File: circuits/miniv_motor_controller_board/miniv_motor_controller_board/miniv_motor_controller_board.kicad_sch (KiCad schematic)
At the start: 25 parts, among them J1 DC_in, J2 T200_ESC_power, J3 T200_ESC_signal, J4 Conn_EStop_Signal, Q1 2SC1815, Q2 2SC1815, U1 Teensy4.1, U2 TLP222A, U3 TLP222A

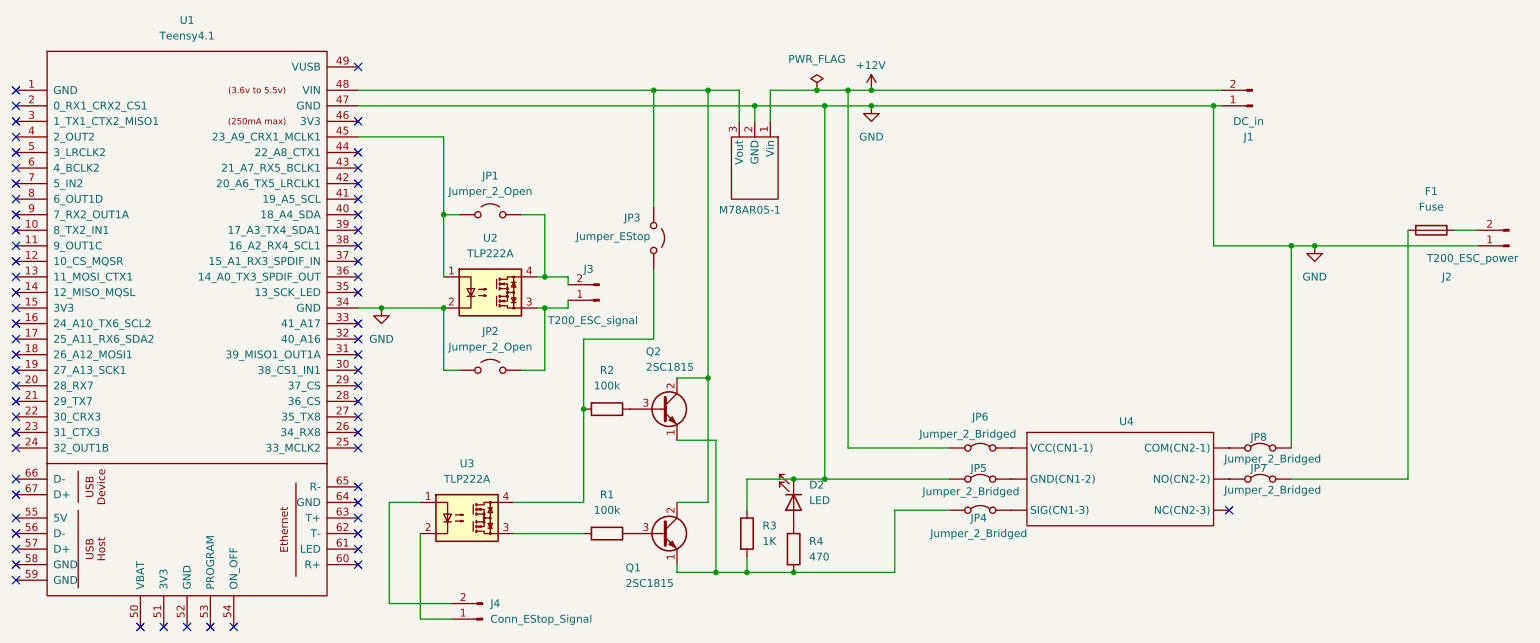
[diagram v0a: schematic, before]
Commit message: modify resister
Signed-off-by: Masaya Kataoka <ms.kataoka@gmail.com>
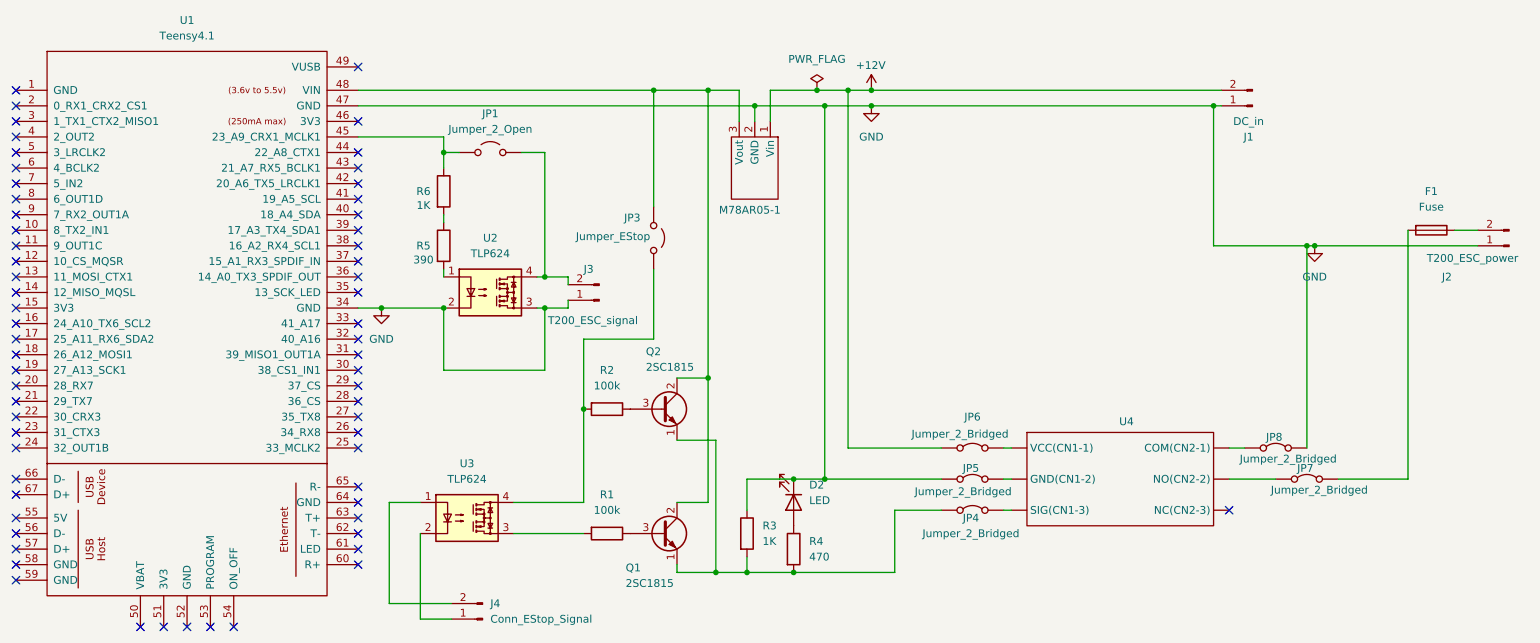
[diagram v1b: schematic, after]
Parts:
- removed JP2: Jumper_2_Open, Connector_PinHeader_2.54mm:PinHeader_1x02_P2.54mm_Vertical, symbol Jumper:Jumper_2_Open
- added R5: 390, Resistor_THT:R_Axial_DIN0207_L6.3mm_D2.5mm_P10.16mm_Horizontal, symbol Device:R
- added R6: 1K, Resistor_THT:R_Axial_DIN0207_L6.3mm_D2.5mm_P10.16mm_Horizontal, symbol Device:R
- J3: footprint (none) -> Connector_AMASS:AMASS_XT30PW-F_1x02_P2.50mm_Horizontal
- M78AR05-1: footprint (none) -> M78AR05-1:M78AR05-1
- U2, U3: value TLP222A -> TLP624
- U4: footprint (none) -> AE-RELAY953B-12V:AE-RELAY953B-12V
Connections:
- net GND: now also J3.1 (Pin_1), U2.3
- net at JP1.1 (A), U1.45 (23_A9_CRX1_MCLK1): now also R6.1; no longer U2.1
- net at U4. (VCC(CN1-1)): now also JP7.1 (A)
- new net: R5.2, U2.1
- new net: R5.1, R6.2
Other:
- moved on the sheet: JP1, JP4, JP5, JP6, JP7, JP8
